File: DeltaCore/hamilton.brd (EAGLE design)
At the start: 45 x 41.5 mm, 69 parts, among them Q3 MOSFET-NCHANNEL_SOT23-3, Q4 MOSFET-NCHANNEL_SOT23-3, Q5 MOSFET-NCHANNEL_SOT23-3, Q6 MOSFET-NCHANNEL_SOT23-3, Q7 NFET_AON7408, Q8 NFET_AON7408, U1 SAMR21, U10 PCA9557, U3 MMA7660FC, U4 AT30TS74, U5 MCP73871-2AAI/ML, U7 BQ29718, U8 MCP1824ST-3302E/DB, U9 TPS61090, X1 XTAL

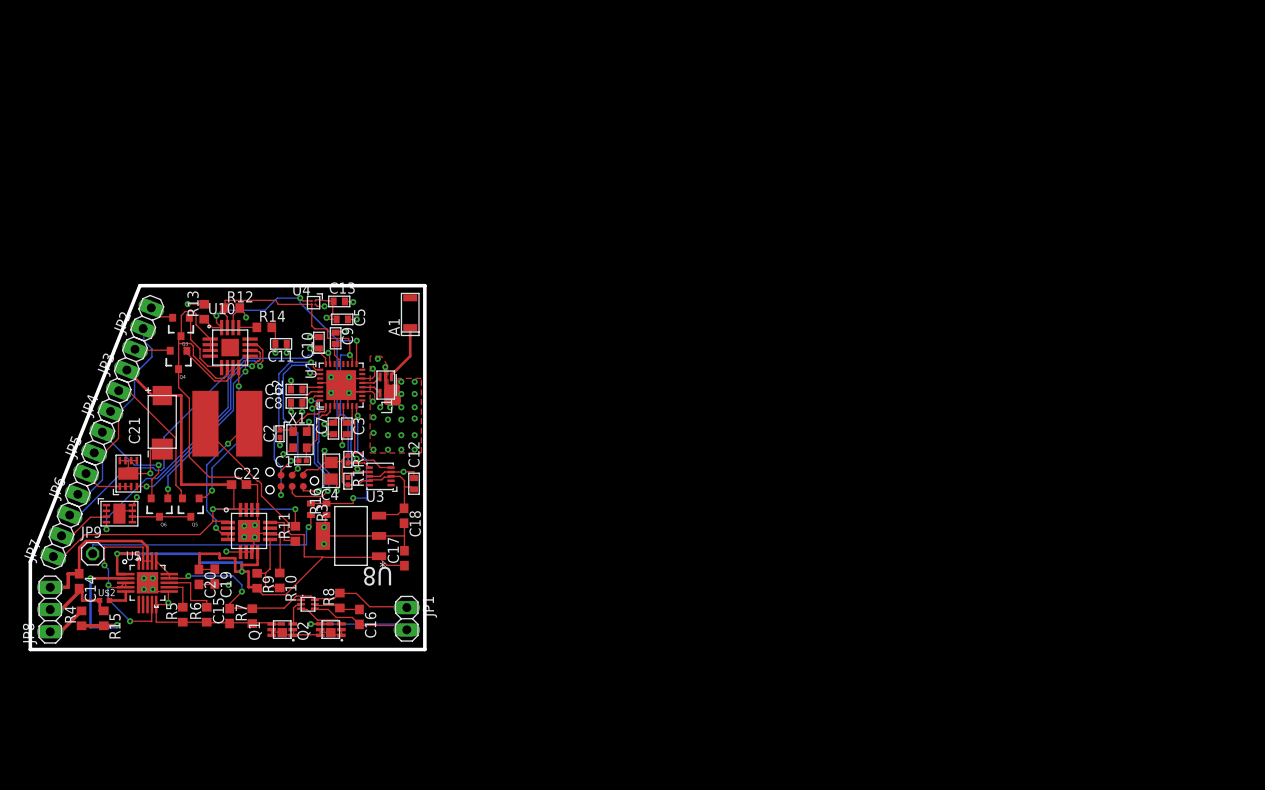
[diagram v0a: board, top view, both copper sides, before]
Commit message: todos
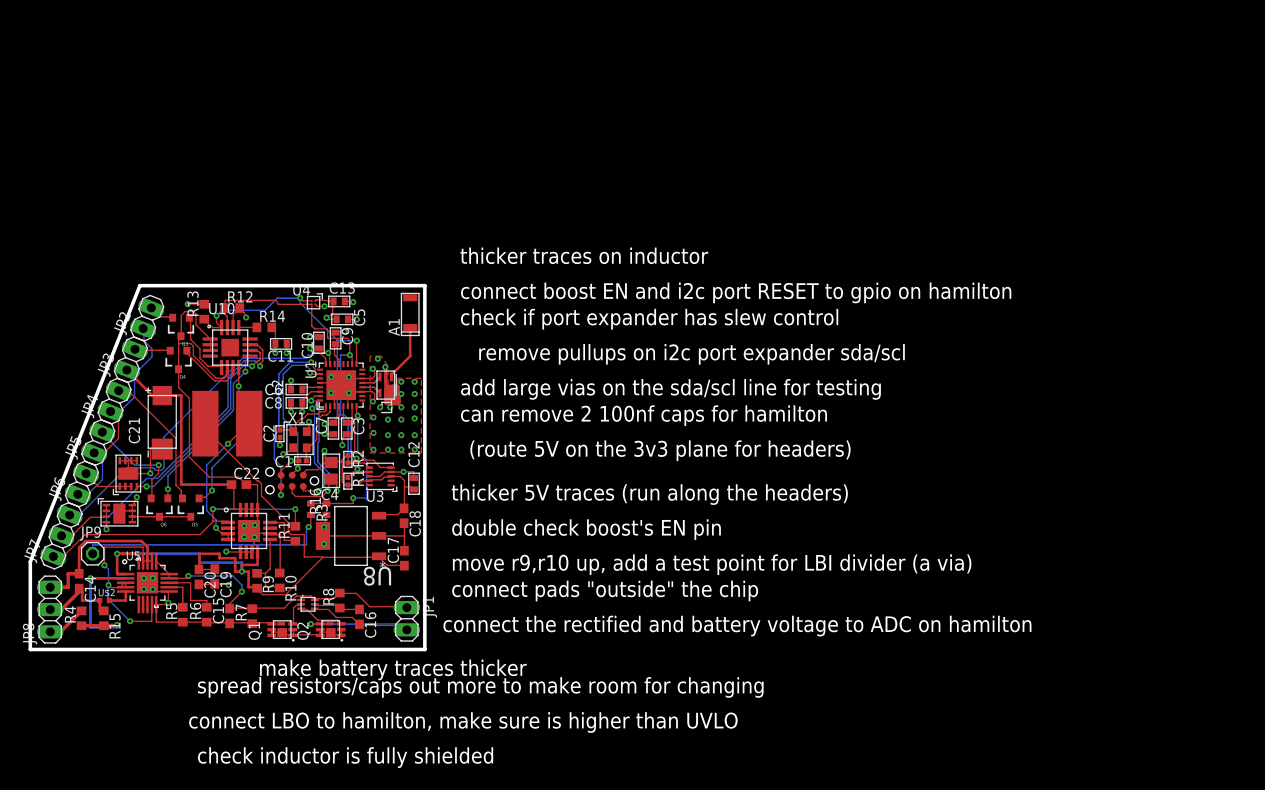
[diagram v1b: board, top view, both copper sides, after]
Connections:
- removed net LS: U1.9
- net OOB: no longer U1.25
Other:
- board text added: "(route 5V on the 3v3 plane for headers)"
- board text added: "add large vias on the sda/scl line for testing"
- board text added: "can remove 2 100nf caps for hamilton"
- board text added: "check if port expander has slew control"
- board text added: "check inductor is fully shielded"
- board text added: "connect LBO to hamilton, make sure is higher than UVLO"
- board text added: "connect boost EN and i2c port RESET to gpio on hamilton"
- board text added: "connect pads "outside" the chip"
- board text added: "connect the rectified and battery voltage to ADC on hamilton"
- board text added: "double check boost's EN pin"
- board text added: "make battery traces thicker"
- board text added: "move r9,r10 up, add a test point for LBI divider (a via)"
- board text added: "remove pullups on i2c port expander sda/scl"
- board text added: "spread resistors/caps out more to make room for changing"
- board text added: "thicker 5V traces (run along the headers)"
- board text added: "thicker traces on inductor"
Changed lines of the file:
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@@
 <?xml version="1.0" encoding="utf-8"?>
 <!DOCTYPE eagle SYSTEM "eagle.dtd">
-<eagle version="7.6.0">
+<eagle version="7.4.0">
 <drawing>
 <settings>
@@
 <setting verticaltext="up"/>
 </settings>
-<grid distance="10" unitdist="mil" unit="mil" style="lines" multiple="1" display="yes" altdistance="0.000000123031" altunitdist="inch" altunit="inch"/>
+<grid distance="1" unitdist="mm" unit="mm" style="lines" multiple="1" display="yes" altdistance="0.000000123031" altunitdist="inch" altunit="inch"/>
 <layers>
 <layer number="1" name="Top" color="4" fill="1" visible="yes" active="yes"/>
@@
 <layer number="27" name="tValues" color="7" fill="1" visible="no" active="yes"/>
 <layer number="28" name="bValues" color="7" fill="1" visible="no" active="yes"/>
-<layer number="29" name="tStop" color="7" fill="3" visible="no" active="yes"/>
+<layer number="29" name="tStop" color="7" fill="3" visible="yes" active="yes"/>
 <layer number="30" name="bStop" color="7" fill="6" visible="no" active="yes"/>
 <layer number="31" name="tCream" color="7" fill="4" visible="no" active="yes"/>
@@
 <wire x1="12.5" y1="41.5" x2="45" y2="41.5" width="0.4064" layer="20"/>
 <wire x1="45" y1="41.5" x2="45" y2="0" width="0.4064" layer="20"/>
+<text x="19" y="-5" size="1.778" layer="20">spread resistors/caps out more to make room for changing</text>
+<text x="26" y="-3" size="1.778" layer="20">make battery traces thicker</text>
+<text x="18" y="-9" size="1.778" layer="20">connect LBO to hamilton, make sure is higher than UVLO</text>
+<text x="48" y="9" size="1.778" layer="20">move r9,r10 up, add a test point for LBI divider (a via)</text>
+<text x="48" y="6" size="1.778" layer="20">connect pads "outside" the chip</text>
+<text x="48" y="13" size="1.778" layer="20">double check boost's EN pin</text>
+<text x="48" y="17" size="1.778" layer="20">thicker 5V traces (run along the headers)</text>
+<text x="50" y="22" size="1.778" layer="20">(route 5V on the 3v3 plane for headers)</text>
+<text x="49" y="26" size="1.778" layer="20">can remove 2 100nf caps for hamilton</text>
+<text x="49" y="29" size="1.778" layer="20">add large vias on the sda/scl line for testing</text>
+<text x="51" y="33" size="1.778" layer="20">remove pullups on i2c port expander sda/scl</text>
+<text x="49" y="37" size="1.778" layer="20">check if port expander has slew control</text>
+<text x="49" y="40" size="1.778" layer="20">connect boost EN and i2c port RESET to gpio on hamilton</text>
+<text x="49" y="44" size="1.778" layer="20">thicker traces on inductor</text>
+<text x="47" y="2" size="1.778" layer="20">connect the rectified and battery voltage to ADC on hamilton</text>
+<text x="19" y="-13" size="1.778" layer="20">check inductor is fully shielded</text>
 </plain>
 <attributes>
@@
 <wire x1="36.4236" y1="34.9758" x2="36.449" y2="33.5788" width="0.1524" layer="1"/>
 </signal>
-<signal name="LS">
-<contactref element="U1" pad="9"/>
-</signal>
 <signal name="ACC">
 <contactref element="U3" pad="5"/>
@@
 </signal>
 <signal name="OOB">
-<contactref element="U1" pad="25"/>
 <contactref element="U$1" pad="6"/>
-<wire x1="33.058" y1="31.912" x2="32.565" y2="31.912" width="0.1524" layer="1"/>
 <wire x1="32.565" y1="31.912" x2="32.283" y2="32.194" width="0.1524" layer="1"/>
 <wire x1="32.283" y1="32.194" x2="32.283" y2="32.448" width="0.1524" layer="1"/>

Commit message: fixes
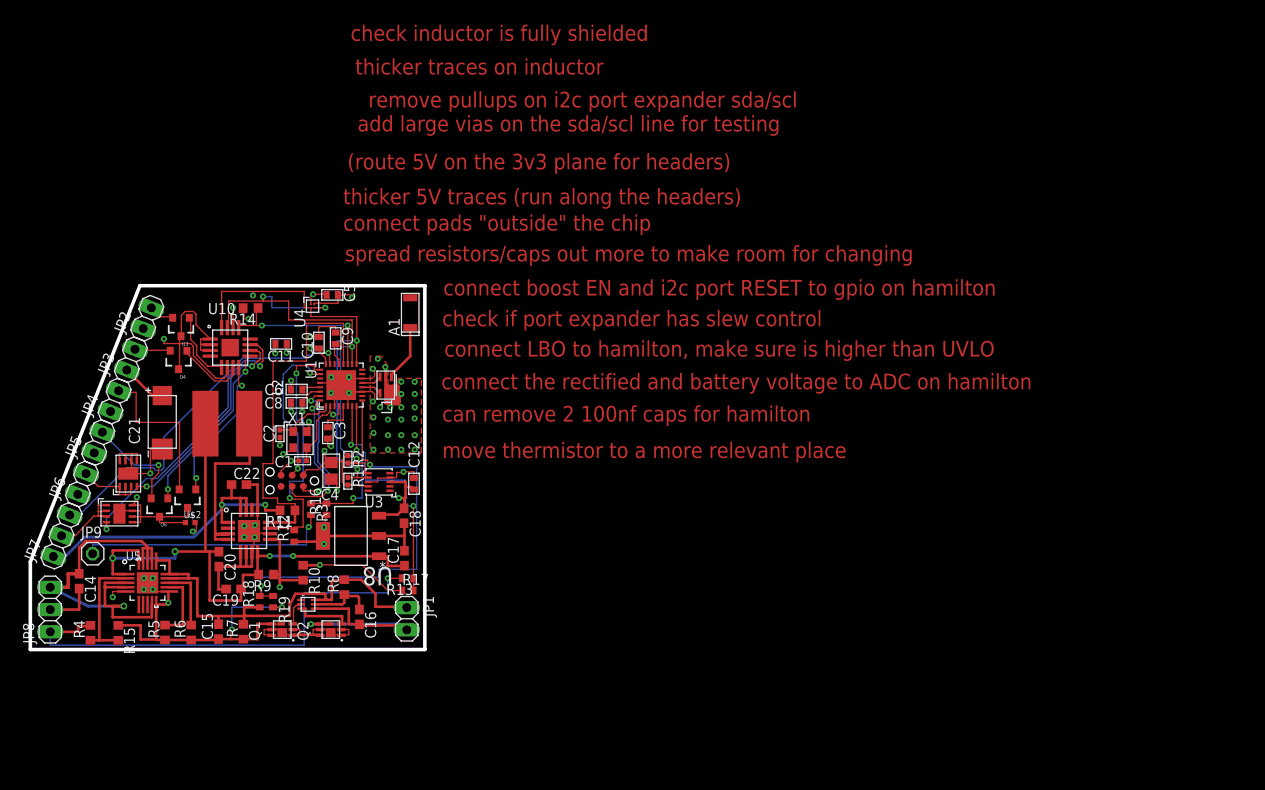
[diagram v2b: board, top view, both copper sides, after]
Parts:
- removed C13, C7: 100nF, storm:C0402
- added R17: 2k, resistor:R0402
- added R18: 13k, resistor:R0402
- added R19: 5k, resistor:R0402
- R12: value 1.6k -> 10k; device resistor:R0603 -> resistor:R0402
- R13: value 1.6k -> 68k; device resistor:R0603 -> resistor:R0402
- R14: value 1.1k -> 10k
- moved R13 38.3 mm to (43.1, 8.13), turned to 180 degrees
- moved R12 26.9 mm to (30.1, 13.0), turned to 90 degrees
- moved U$2 13.2 mm to (18.2, 14.5)
- moved C20 3.06 mm to (21.5, 10.3)
- moved C5 3.02 mm to (34.4, 40.4)
- moved R5 2.87 mm to (15.4, 1.94)
- moved R11 2.81 mm to (29.3, 15.9), turned to 180 degrees
- moved R10 2.81 mm to (31.1, 8.76)
- moved R14 2.70 mm to (25.1, 38.9), turned to 180 degrees
- moved R6 2.70 mm to (18.3, 1.94)
- moved C19 2.57 mm to (23.2, 6.90), turned to 180 degrees
- moved R15 2.33 mm to (10.0, 1.91)
- moved C3 2.22 mm to (33.9, 24.7)
- moved C15 2.18 mm to (21.5, 2.04)
- moved R7 2.05 mm to (24.3, 2.03)
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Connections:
- removed net N$29: R14.1, U10.P$13
- new net BAT: R18.2, R19.1, U1.9
- new net EN: R12.2, U1.25, U9.EN
- new net N$12: U1.10
- new net N$15: U1.15
- new net N$17: U1.16
- new net N$42: U1.22
- new net RST: R14.1, U1.19, U10.P$13
- new net WIT: R13.1, R17.2, U1.7
- net +3V3: no longer C13.1, C7.1, R12.2, R13.2, R14.2
- net ACC: no longer U1.7
- net GND: now also R12.1, R14.2, R17.1, R19.2; no longer C13.2, C7.2
- net LBO: now also U1.20
- net N$1: now also JP8.1, R13.2, R4.2; no longer R15.2, R4.1, U5.2
- net N$20: now also R18.1
- net RECT: now also R15.2, R4.1, U5.2; no longer JP8.1, R4.2
- net SCL: no longer R12.1
- net SDA: no longer R13.1
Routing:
- net 5V: track 93.5 -> 45.2 mm
- net BAT: track 0.00 -> 47.9 mm, vias 0 -> 2
- net LBO: track 5.15 -> 43.1 mm
- net N$1: track 17.1 -> 54.6 mm, vias 2 -> 1
- net GND: track 210.9 -> 248.2 mm, vias 59 -> 58
- net EN: track 0.00 -> 29.9 mm, vias 0 -> 2
- net WIT: track 0.00 -> 28.3 mm, vias 0 -> 2
- net OOB: track 20.6 -> 0.00 mm, vias 2 -> 0
- net RST: track 0.00 -> 19.3 mm, vias 0 -> 2
- net N$19: track 2.92 -> 20.3 mm, vias 0 -> 2
- net N$20: track 36.9 -> 50.4 mm, vias 2 -> 0
- net +3V3: track 52.8 -> 40.1 mm
- net OUT: track 83.6 -> 71.2 mm, vias 2 -> 4
- net SCL: track 42.6 -> 54.8 mm, vias 2 -> 4
- net ACC: track 10.8 -> 0.00 mm
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- added copper zone on layer 15, net 5V
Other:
- board text added: "move thermistor to a more relevant place"
- board text removed: "double check boost's EN pin"
- board text removed: "make battery traces thicker"
- board text removed: "move r9,r10 up, add a test point for LBI divider (a via)"

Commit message: more
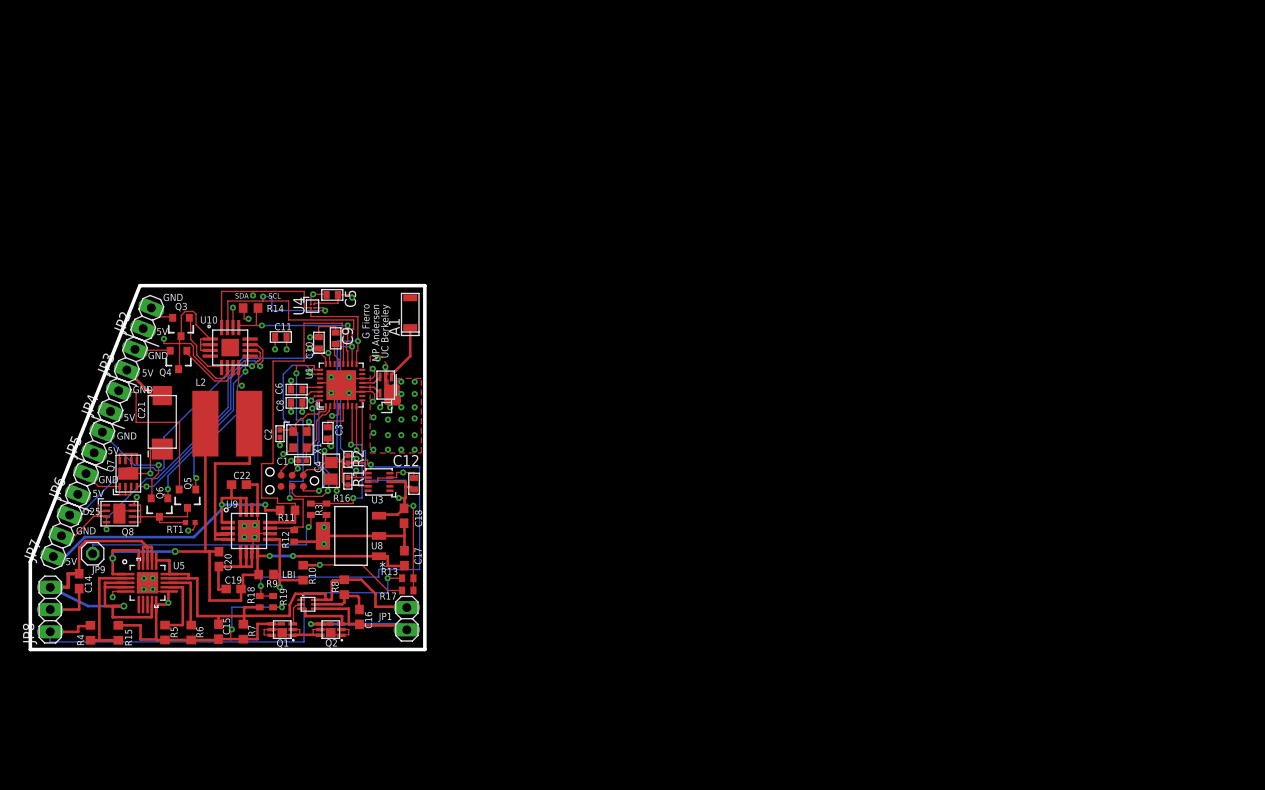
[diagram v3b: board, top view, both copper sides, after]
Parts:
- moved C11 0.79 mm to (28.6, 35.6)
- renumbered U$2 to RT1
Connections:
- removed net ACC: U3.5
- removed net OOB: U$1.6
- removed net SD: U1.27
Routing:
- net SCL: track 54.8 -> 55.7 mm
- net N$1: track 54.6 -> 53.9 mm
- net BAT: track 47.9 -> 48.6 mm
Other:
- board text added: "5V"
- board text added: "D25"
- board text added: "G Fierro"
- board text added: "GND"
- board text added: "LBI"
- board text added: "MP Andersen"
- board text added: "Q7"
- board text added: "Q8"
- board text added: "SCL"
- board text added: "SDA"
- board text added: "UC Berkeley"
- board text removed: "(route 5V on the 3v3 plane for headers)"
- board text removed: "add large vias on the sda/scl line for testing"
- board text removed: "can remove 2 100nf caps for hamilton"
- board text removed: "check if port expander has slew control"
- board text removed: "check inductor is fully shielded"
- board text removed: "connect LBO to hamilton, make sure is higher than UVLO"
- board text removed: "connect boost EN and i2c port RESET to gpio on hamilton"
- board text removed: "connect pads "outside" the chip"
- board text removed: "connect the rectified and battery voltage to ADC on hamilton"
- board text removed: "move thermistor to a more relevant place"
- board text removed: "remove pullups on i2c port expander sda/scl"
- board text removed: "spread resistors/caps out more to make room for changing"
- board text removed: "thicker 5V traces (run along the headers)"
- board text removed: "thicker traces on inductor"
